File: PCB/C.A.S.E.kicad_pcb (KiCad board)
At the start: 4 copper layers, 106.3 x 121.1 mm, 49 parts, among them J1 CQ-USB-C16PSMT01, J2 Conn_01x02_Pin, J3 Conn_02x04_Top_Bottom, SW1 SW_Push, SW12 SW_SPDT, SW13 RotaryEncoder_Switch, SW2 SW_Push, SW3 SW_Push, SW4 SW_Push, SW5 SW_Push, SW6 SW_Push, SW7 SW_Push, SW8 SW_Push, U2 AP2112K-3.3, U3 BQ24072TRGTR, X1 ESP32-S3-WROOM-1-N16R8

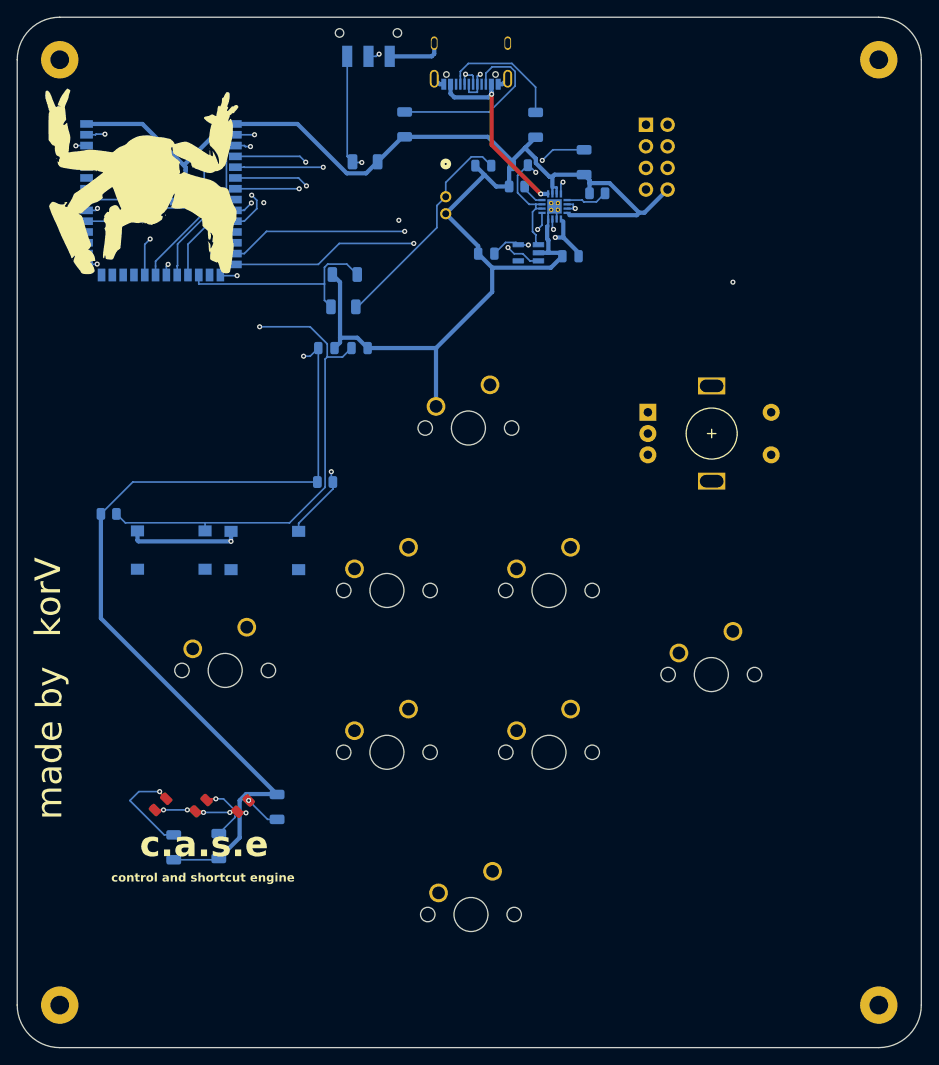
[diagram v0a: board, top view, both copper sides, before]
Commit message: changed everything
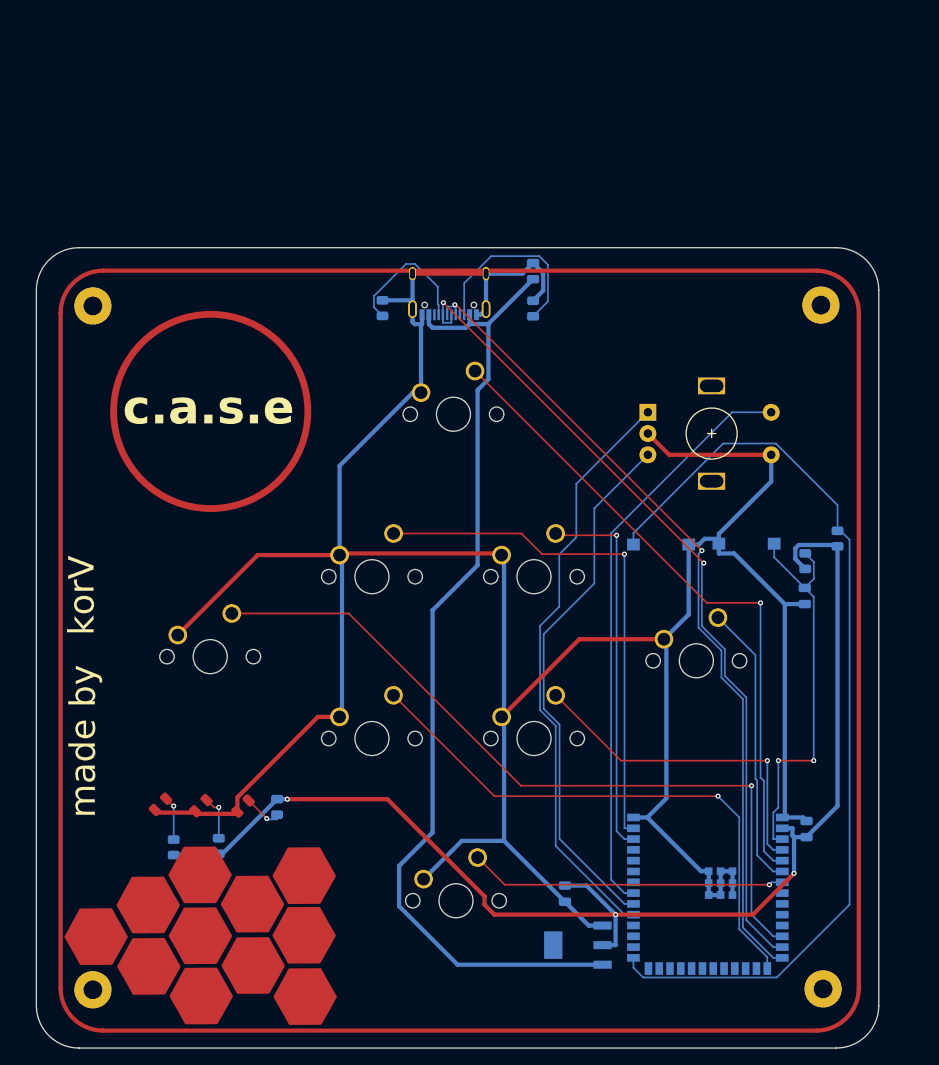
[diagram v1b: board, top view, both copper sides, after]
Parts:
- removed C3: 4.7uF, LED_SMD:LED_0805_2012Metric
- removed C4: 1uF, Capacitor_SMD:C_1206_3216Metric
- removed C5: 10uF, Capacitor_SMD:C_0805_2012Metric
- removed the G*** at (129.6, 58.1)
- removed the G*** at (186.4, 156.0)
- removed the G*** at (183.8, 146.2)
- removed J2: Conn_01x02_Pin, All components:CONN_S2B-PH-K-S_JST
- removed J3: Conn_02x04_Top_Bottom, Connector_PinHeader_2.54mm:PinHeader_2x04_P2.54mm_Vertical
- removed R3: 3.3k, Resistor_SMD:R_0805_2012Metric
- removed R4: 1.8k, Resistor_SMD:R_1206_3216Metric
- removed R5: 10k, Resistor_SMD:R_0805_2012Metric
- removed R8, R9: 100k, Resistor_SMD:R_1206_3216Metric
- removed REF**: OSHW-Logo_5.7x6mm_SilkScreen, Symbol:OSHW-Logo_5.7x6mm_SilkScreen
- removed SW12: SW_SPDT, All components:SW_JS102011SAQN
- removed U2: AP2112K-3.3, All components:SOT95P285X140-5N
- removed U3: BQ24072TRGTR, All components:RGT16_1P7X1P7
- removed boot1, rst1: SW_Push, All components:SW_PTS645SL43SMTR92LFS
- added ?: LOGO, LOGO, F.Cu at (141.3, 143.9)
- added ?: LOGO, LOGO, F.Cu at (135.1, 147.6)
- added ?: LOGO, LOGO, F.Cu at (135.1, 140.5)
- added ?: LOGO, LOGO, F.Cu at (135.2, 154.7)
- added ?: LOGO, LOGO, F.Cu at (147.3, 147.6)
- added ?: LOGO, LOGO, F.Cu at (122.9, 147.7)
- added ?: LOGO, LOGO, F.Cu at (129.0, 144.0)
- added ?: LOGO, LOGO, F.Cu at (147.3, 140.6)
- added ?: LOGO, LOGO, F.Cu at (141.3, 151.1)
- added ?: LOGO, LOGO, F.Cu at (129.1, 151.2)
- added ?: LOGO, LOGO, F.Cu at (147.5, 154.8)
- added U1: TLV1117-33, All components:SOT230P700X180-4N, B.Cu at (179.6, 148.8)
- added boot: SW_Push, All components:434121025816, B.Cu at (189.3, 101.7)
- added rst: SW_Push, All components:434121025816, B.Cu at (199.4, 101.6)
- C2: value 4.7uF -> 10uF; footprint LED_SMD:LED_0805_2012Metric -> Capacitor_SMD:C_0805_2012Metric
- R1, R2: footprint Resistor_SMD:R_1206_3216Metric -> Resistor_SMD:R_0805_2012Metric
- R10: value 68 -> 150; footprint Resistor_SMD:R_1206_3216Metric -> Resistor_SMD:R_0805_2012Metric
- R11, R12: value 33 -> 150; footprint Resistor_SMD:R_1206_3216Metric -> Resistor_SMD:R_0805_2012Metric
- moved X1 103.8 mm to (194.8, 139.1)
- moved C2 85.8 mm to (178.1, 142.8), turned to -90 degrees
- moved R6 82.1 mm to (206.3, 103.7), turned to -90 degrees
- moved C6 79.9 mm to (206.4, 135.2), turned to -90 degrees
- moved R7 60.6 mm to (210.1, 101.0), turned to -90 degrees
- moved C7 59.9 mm to (206.2, 107.8), turned to 90 degrees
- moved H4 29.6 mm to (208.2, 73.5)
- moved H3 29.2 mm to (122.5, 73.7)
- moved R2 28.1 mm to (156.6, 73.9), turned to -90 degrees
- moved J1 27.2 mm to (164.4, 74.7)
- moved R1 26.4 mm to (174.3, 74.0), turned to 90 degrees
- moved H1 6.82 mm to (208.4, 153.9)
- moved C1 4.74 mm to (174.3, 69.5), turned to 90 degrees
- moved H2 4.30 mm to (122.5, 154.1)
- moved SW3 2.39 mm to (157.9, 119.4)
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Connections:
- C1 pad 1: GND -> VBUS
- C1 pad 2: VBUS -> GND
- C2 pad 1: /VSYS -> +3.3V
- X1 pad 18: /pgood -> unconnected-(X1-IO10-Pad18)
- X1 pad 19: /chg_detection -> unconnected-(X1-IO11-Pad19)
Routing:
- net GND: track 486.6 -> 373.3 mm, vias 6 -> 0
- net VBUS: track 34.7 -> 116.6 mm, vias 3 -> 0
- net /busy: track 75.6 -> 0.00 mm, vias 1 -> 0
- net /dc: track 71.7 -> 0.00 mm, vias 1 -> 0
- net /btn_6: track 104.6 -> 33.6 mm, vias 2 -> 0
- net /res: track 69.8 -> 0.00 mm, vias 1 -> 0
- net /boot: track 47.7 -> 111.0 mm, vias 2 -> 0
- net /btn_7: track 97.2 -> 37.3 mm
- net /cs: track 56.6 -> 0.00 mm, vias 1 -> 0
- net /chg_detection: track 55.4 -> 0.00 mm, vias 2 -> 0
- net /pgood: track 54.0 -> 0.00 mm, vias 2 -> 0
- net /scl: track 53.2 -> 0.00 mm, vias 1 -> 0
- net /sda: track 52.8 -> 0.00 mm, vias 1 -> 0
- net /USB_D-: track 45.6 -> 97.4 mm
- net /VSYS: track 49.1 -> 0.00 mm, vias 2 -> 0
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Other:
- board size 106.3 x 121.1 mm -> 99 x 94.1 mm
- copper layers 4 -> 2
- board text added: "150"
- board text removed: "10uF"
- board text removed: "33"
- board text removed: "68"
- board text removed: "boot"
- board text removed: "control and shortcut engine"
- board text removed: "rst"
